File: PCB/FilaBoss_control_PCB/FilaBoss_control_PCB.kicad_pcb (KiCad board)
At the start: 2 copper layers, 102.9 x 87.6 mm, 52 parts, among them J1 Encoder, J10 Power 3.3v, J11 SDA/SCL, J12 power 12v, J13 power 5v, J14 Fan connector, J15 power 24v, J16 Load, J17 manual, J18 Control leds, J2 SPOOL, J3 PULLER, J4 Conn_01x02_Pin, J5 Power, J6 INA219, J7 Stepper, J8 limit switch, J9 Extruder, Q1 IRLZ44N, Q2 IRLZ44N, U2 R-78E5.0-0.5, U4 R-78E12-2

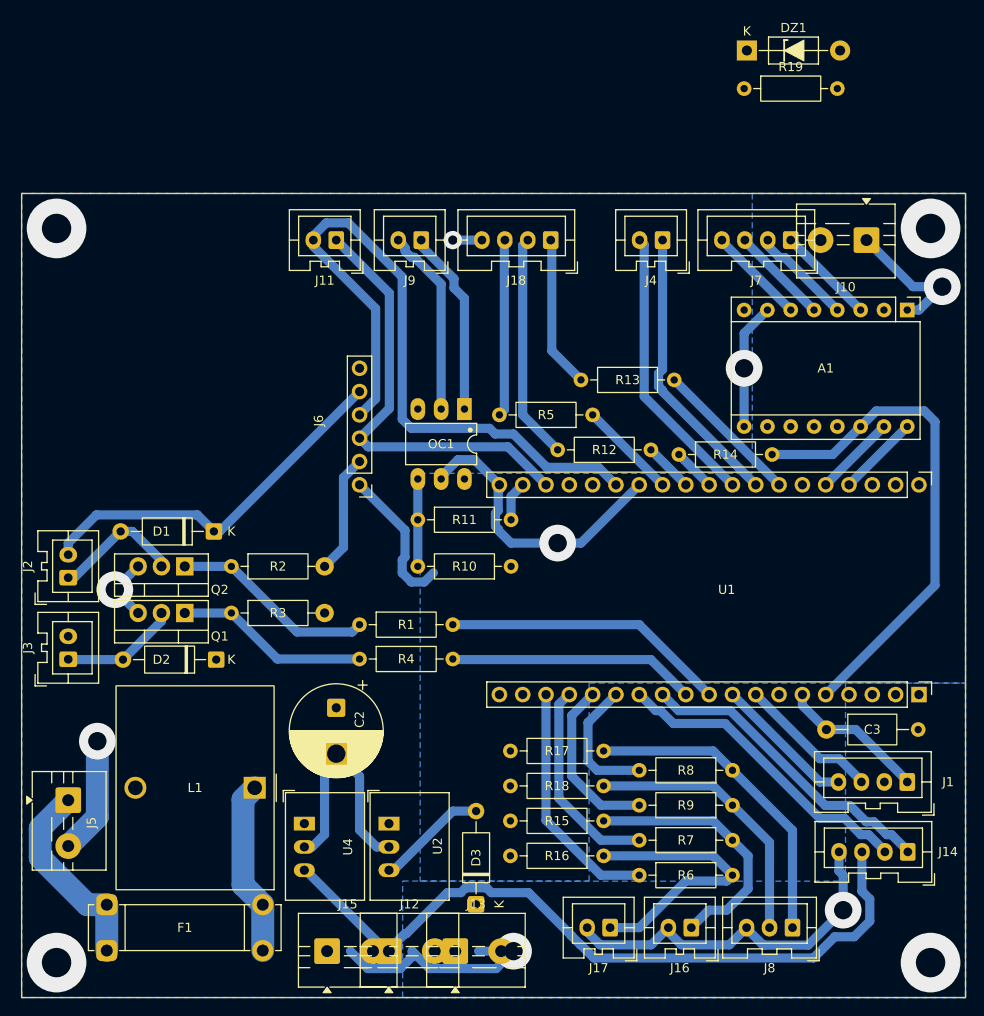
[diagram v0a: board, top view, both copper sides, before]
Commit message: pcb v3
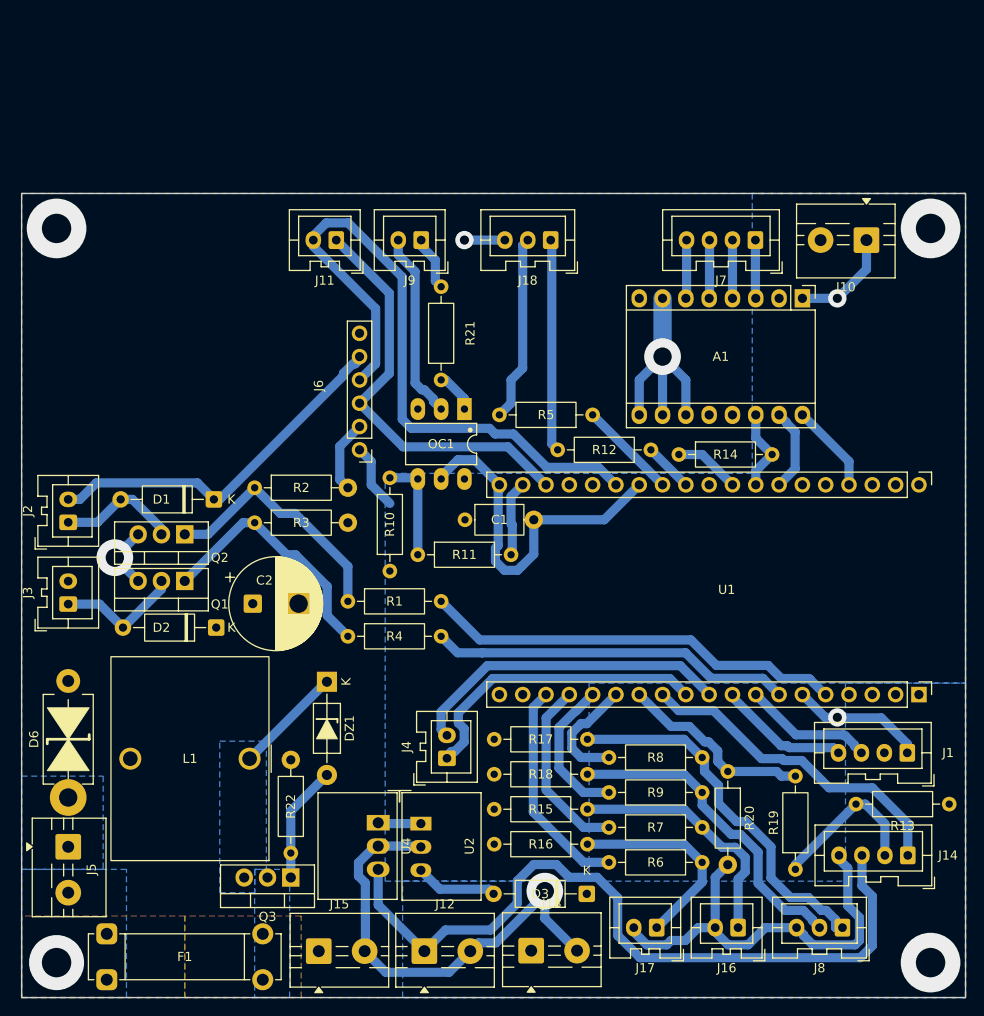
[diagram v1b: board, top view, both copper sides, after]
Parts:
- removed C3: C, Capacitor_THT:C_Axial_L5.1mm_D3.1mm_P10.00mm_Horizontal
- added C1: C, Capacitor_THT:C_Axial_L5.1mm_D3.1mm_P7.50mm_Horizontal, F.Cu at (86.4, 121.9)
- added D6: 1.5KE36CA, PCM_Diode_THT_AKL:D_DO-201_P12.70mm_Horizontal_TVS, F.Cu at (43.2, 152.2)
- added Q3: IRF9540N, PCM_Package_TO_SOT_THT_AKL:TO-220-3_Vertical_GDS, F.Cu at (67.4, 160.9)
- added R20: 2k, Resistor_THT:R_Axial_DIN0207_L6.3mm_D2.5mm_P10.16mm_Horizontal, F.Cu at (115.1, 149.4)
- added R21: 4.7k, Resistor_THT:R_Axial_DIN0207_L6.3mm_D2.5mm_P10.16mm_Horizontal, F.Cu at (83.8, 106.7)
- added R22: 2k, Resistor_THT:R_Axial_DIN0207_L6.3mm_D2.5mm_P10.16mm_Horizontal, F.Cu at (67.4, 148.1)
- DZ1: value 1N4728A -> 1EZ15
- J18: footprint Connector_JST:JST_XA_B04B-XASK-1_1x04_P2.50mm_Vertical -> Connector_JST:JST_XA_B03B-XASK-1_1x03_P2.50mm_Vertical
- J4: value Conn_01x02_Pin -> RX/TX
- R12, R5: value 220R -> 330R
- R19: value 330R -> 1k
- U4: value R-78E12-2 -> R-78B12-2.0; footprint Converter_DCDC:Converter_DCDC_RECOM_R-78E-0.5_THT -> Converter_DCDC:Converter_DCDC_RECOM_R-78B-2.0_THT
- moved R19 85.3 mm to (122.4, 160.0), turned to 90 degrees
- moved DZ1 82.6 mm to (71.4, 139.6), turned to -90 degrees
- moved J4 61.2 mm to (84.5, 147.9), turned to 90 degrees
- moved R13 55.1 mm to (139.2, 152.9)
- moved C2 14.5 mm to (63.3, 131.1), turned to 0 degrees
- moved R10 13.2 mm to (78.2, 127.5), turned to 90 degrees
- moved D3 12.1 mm to (99.7, 162.7), turned to 180 degrees
- moved A1 11.5 mm to (123.2, 97.8)
- moved R3 10.2 mm to (63.5, 122.2)
- moved R2 8.94 mm to (63.5, 118.4)
- moved J13 8.28 mm to (93.6, 168.9)
- moved U4 8.05 mm to (77.0, 154.9)
- moved J2 6.03 mm to (43.2, 122.2)
- moved J3 6.01 mm to (43.2, 131.1)
- moved J8 5.45 mm to (127.6, 166.4)
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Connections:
- DZ1 pad 1: +3.3V -> VCC
- DZ1 pad 2: GND -> Net-(DZ1-A)
- J5 pad 1: LINE -> GND
- J5 pad 2: GND -> LINE
- L1 pad 1: VDC -> VCC
- OC1 pad 1: Net-(J9-Pin_1) -> Net-(OC1-Pad1)
- R1 pad 2: Net-(U1-GPIO26) -> Net-(U1-GPIO13)
- R13 pad 1: +3.3V -> +5V
- R14 pad 1: Net-(U1-GPIO4) -> Net-(U1-GPIO17/TX2)
- R4 pad 2: Net-(U1-GPIO25) -> Net-(U1-GPIO12)
- U1 pad 10: Net-(U1-GPIO26) -> Net-(J4-Pin_2)
- U1 pad 11: Net-(U1-GPIO25) -> Net-(J4-Pin_1)
- U1 pad 23: Net-(A1-STEP) -> Net-(A1-DIR)
- U1 pad 26: Net-(U1-GPIO4) -> Net-(A1-STEP)
- U1 pad 27: Net-(J4-Pin_1) -> Net-(A1-UART)
- U1 pad 28: Net-(J4-Pin_2) -> Net-(U1-GPIO17/TX2)
- U1 pad 5: Net-(A1-UART) -> Net-(U1-GPIO13)
- U1 pad 7: Net-(A1-DIR) -> Net-(U1-GPIO12)
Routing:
- net Net-(U1-GPIO13): track 0.00 -> 46.1 mm
- net Net-(A1-UART): track 54.9 -> 9.09 mm
- net Net-(U1-GPIO12): track 0.00 -> 39.5 mm
- net Net-(U1-GPIO26): track 31.1 -> 0.00 mm
- net Net-(U1-GPIO25): track 27.0 -> 0.00 mm
- net LINE: track 21.9 -> 0.00 mm
- net Net-(U1-GPIO32): track 0.00 -> 21.7 mm
- net Net-(U1-GPIO4): track 20.8 -> 0.00 mm
- net (no net): track 19.3 -> 0.00 mm
- net VDC: track 19.2 -> 0.00 mm
- net Net-(J14-Pin_2): track 33.9 -> 17.3 mm
- net Net-(J9-Pin_1): track 20.4 -> 5.98 mm
- net Net-(DZ1-A): track 0.00 -> 12.8 mm
- net VCC: track 0.00 -> 11.9 mm
- net +3.3V: track 16.0 -> 7.21 mm
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- added copper zone on B.Cu, net GND
- added copper zone on B.Cu, net LINE
- added copper zone on F.Cu, net LINE
- added copper zone on B.Cu, net VCC
- added copper zone on B.Cu, net VDC
- added copper zone on F.Cu, net VDC
